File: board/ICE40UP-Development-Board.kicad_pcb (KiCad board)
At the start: 4 copper layers, 41.9 x 20.3 mm, 60 parts, among them X1 USB4105-GF-A, X2 Conn_01x16, X3 Conn_01x16, X4 Tag-Connect, Y1 48MHz

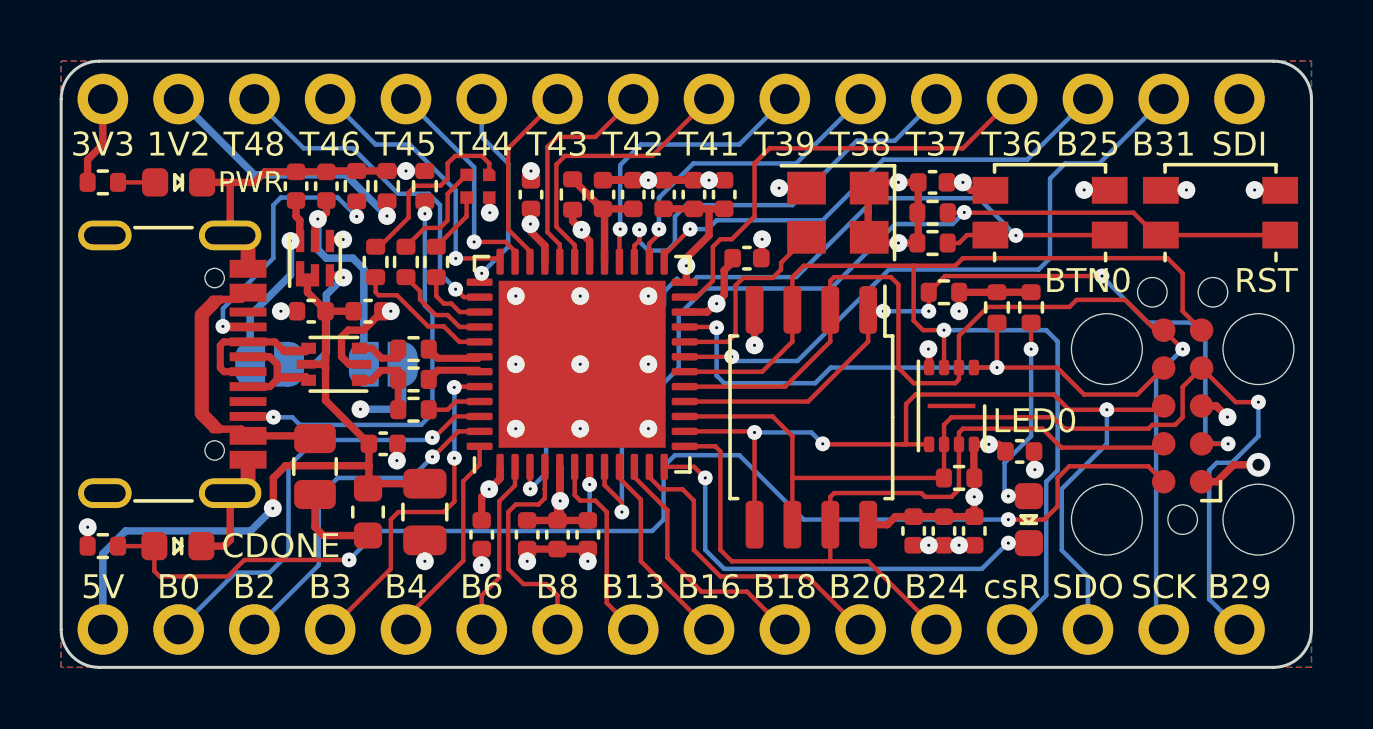
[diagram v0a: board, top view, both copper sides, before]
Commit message: increase size of RAM pads
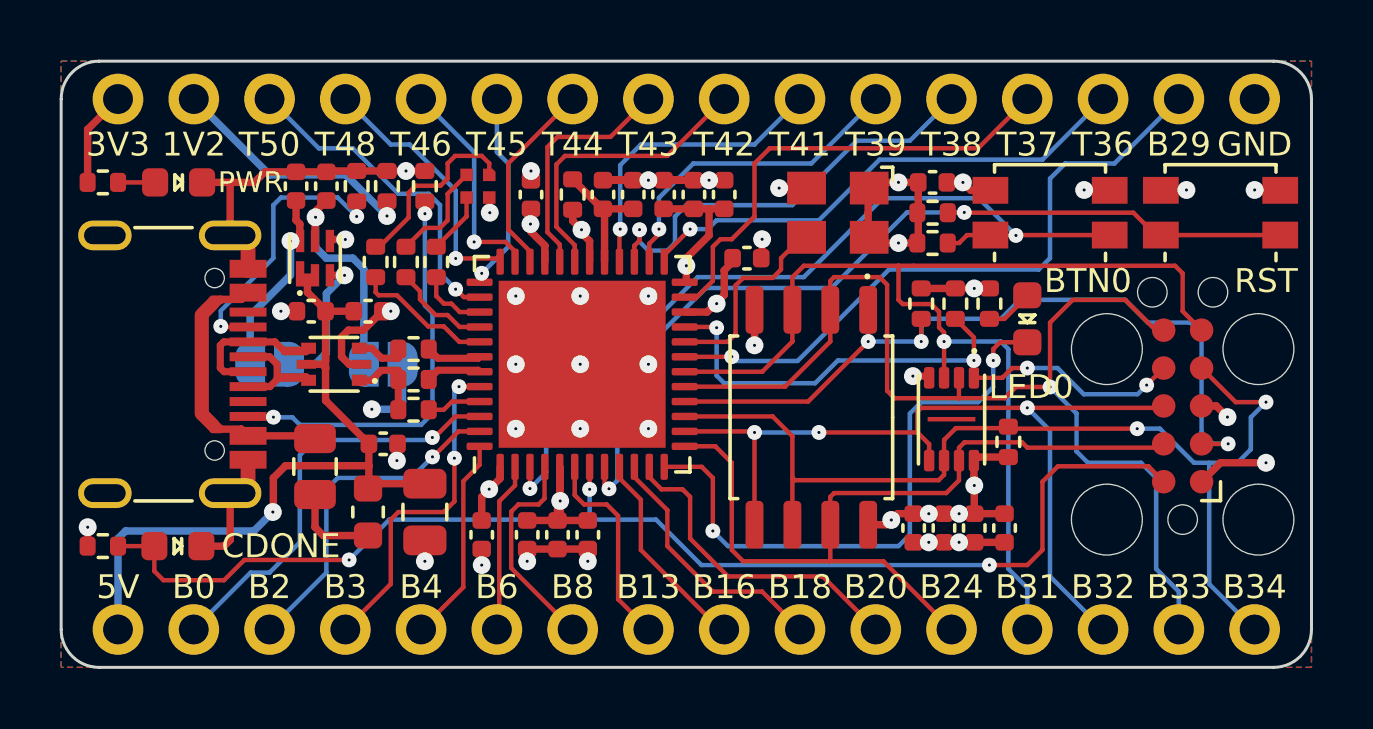
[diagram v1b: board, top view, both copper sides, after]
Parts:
- moved V8 6.73 mm to (78.1, 86.1)
- moved C8 2.62 mm to (77.3, 93.1), turned to 90 degrees
- moved R1 2.05 mm to (77.5, 90.2), turned to 90 degrees
- moved R18 1.40 mm to (76.8, 85.6)
- moved R3 1.40 mm to (75.7, 85.6)
- moved R2 0.85 mm to (74.5, 85.6), turned to -90 degrees
- moved X2 0.51 mm to (47.6, 78.7)
- moved X3 0.51 mm to (47.6, 96.5)
- moved V2 0.44 mm to (75.6, 89.5)
- moved C10 0.10 mm to (76.3, 93.1)
- moved C7 0.10 mm to (74.3, 93.1)
- moved C9 0.10 mm to (75.3, 93.1)
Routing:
- net Net-(V8-A): track 6.92 -> 1.61 mm, vias 2 -> 0
- net CONF_O: track 15.7 -> 20.3 mm
- net SPI_SI: track 35.1 -> 37.2 mm
- net SPI_~{WP}: track 40.4 -> 38.6 mm
- net CDONE: track 43.2 -> 42.2 mm
- net ~{RST}: track 31.6 -> 30.6 mm
- net SPI_~{HOLD}: track 28.7 -> 28.1 mm
- net SPI_SO: track 30.2 -> 29.5 mm
- net IOT_39a: track 10.4 -> 10.9 mm
- net IOT_37b: track 15.4 -> 15.9 mm
- net IOB_0a: track 14.8 -> 14.3 mm
- net IOT_38b: track 14.2 -> 14.8 mm
- net IOT_42b: track 9.54 -> 10.0 mm
- net IOT_50b: track 11.7 -> 11.1 mm
- net IOT_43a: track 7.56 -> 8.07 mm
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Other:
- board text added: "B32"
- board text added: "B33"
- board text added: "B34"
- board text added: "GND"
- board text added: "T50"
- board text removed: "B25"
- board text removed: "SCK"
- board text removed: "SDI"
- board text removed: "SDO"
- board text removed: "csR"
